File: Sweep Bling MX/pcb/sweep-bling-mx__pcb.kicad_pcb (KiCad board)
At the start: 2 copper layers, 113.5 x 95.2 mm, 31 parts, among them J2 AudioJack4dpb, SW10 SW_Push, SW11 SW_Push, SW12 SW_Push, SW14 SW_Push, SW15 SW_Push, SW16 SW_Push, SW17 SW_Push, SW18 SW_Push, SW2 SW_Push, SW20 SW_Push, SW21 SW_Push, SW3 SW_Push, SW4 SW_Push, SW5 SW_Push, SW6 SW_Push, SW8 SW_Push, SW9 SW_Push, U1 ProMicro-kbd

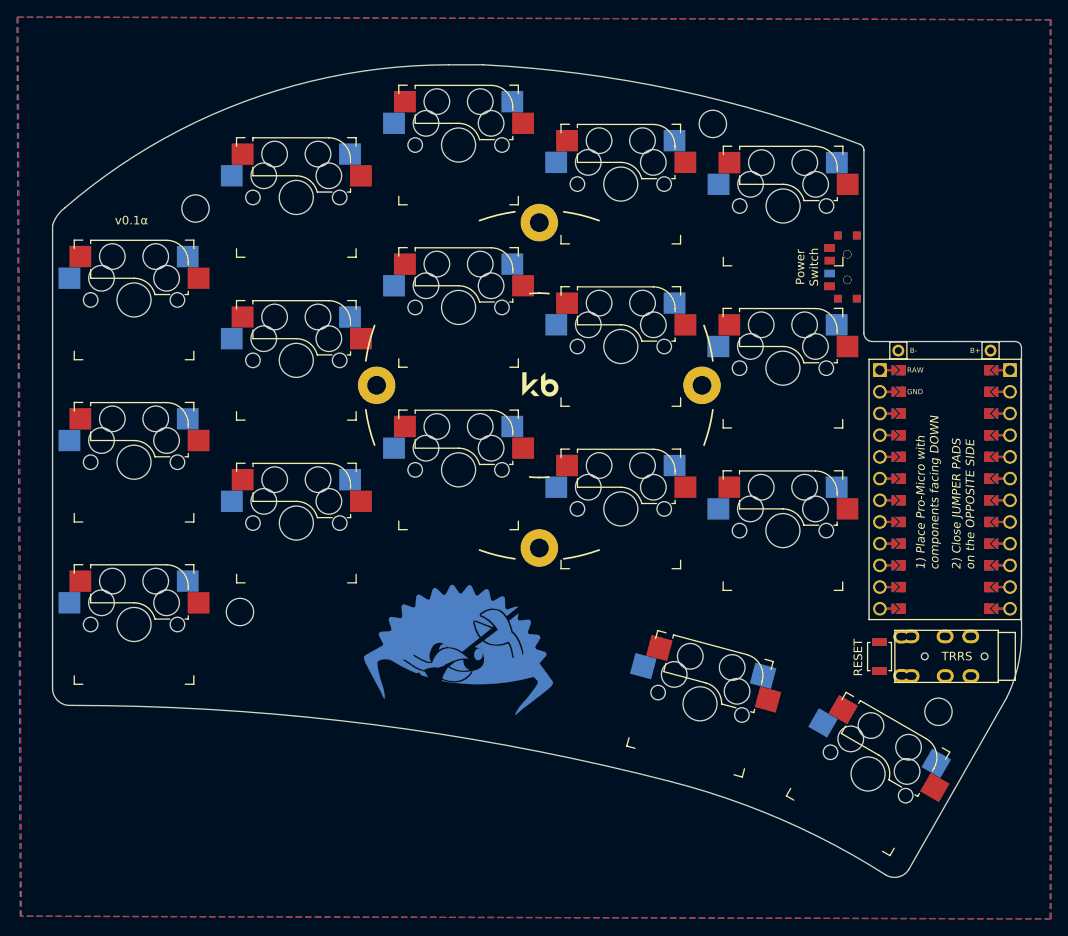
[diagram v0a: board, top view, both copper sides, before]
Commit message: Run auto router
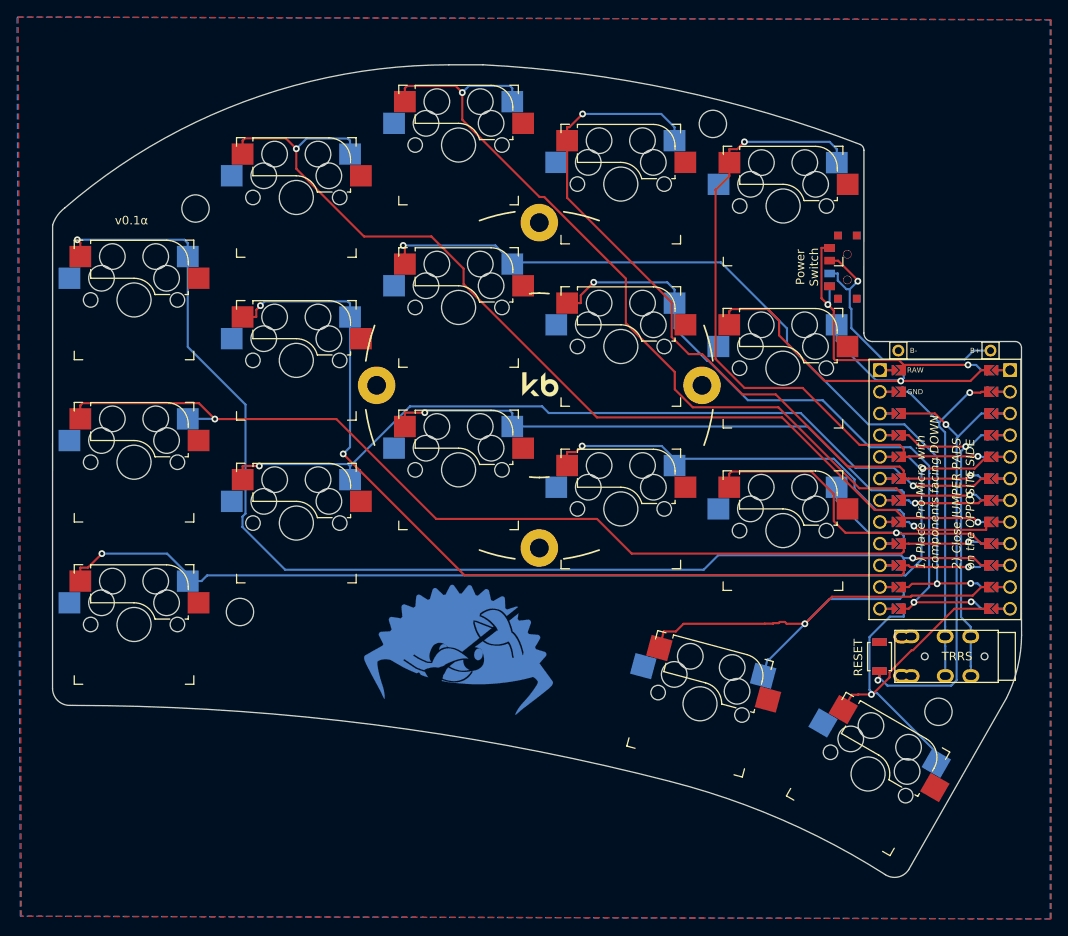
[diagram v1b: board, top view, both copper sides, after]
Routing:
- net Switch1: track 0.00 -> 142.6 mm, vias 0 -> 2
- net Switch11: track 0.00 -> 125.3 mm, vias 0 -> 2
- net Switch6: track 0.00 -> 119.4 mm, vias 0 -> 2
- net Switch2: track 0.00 -> 118.7 mm, vias 0 -> 2
- net Switch7: track 0.00 -> 114.2 mm, vias 0 -> 3
- net Switch3: track 0.00 -> 104.4 mm, vias 0 -> 2
- net Switch8: track 0.00 -> 101.1 mm, vias 0 -> 3
- net Switch12: track 0.00 -> 97.6 mm, vias 0 -> 2
- net Switch4: track 0.00 -> 89.6 mm, vias 0 -> 2
- net Switch9: track 0.00 -> 82.6 mm, vias 0 -> 3
- net Switch5: track 0.00 -> 77.1 mm, vias 0 -> 2
- net Switch13: track 0.00 -> 75.9 mm, vias 0 -> 2
- net Switch16: track 0.00 -> 64.1 mm, vias 0 -> 1
- net Switch14: track 0.00 -> 57.9 mm, vias 0 -> 2
- net reset: track 0.00 -> 52.5 mm, vias 0 -> 2
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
